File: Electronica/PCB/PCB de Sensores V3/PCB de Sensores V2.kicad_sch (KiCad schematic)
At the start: 10 parts, among them J2 Conexion Sensores, U1 ULTRASONICO1, U2 ULTRASONICO2, U3 ULTRASONICO3, U4 ULTRASONICO4, U5 ULTRASONICO5, U6 VL6180 1, U7 VL6180 2

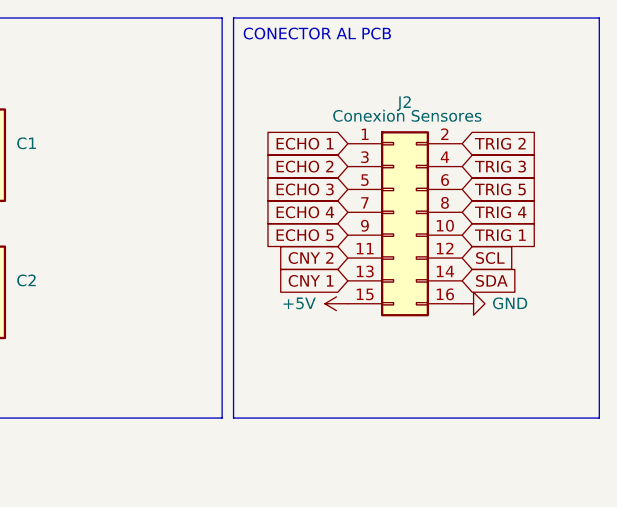
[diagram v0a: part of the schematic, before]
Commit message: Sensores V3
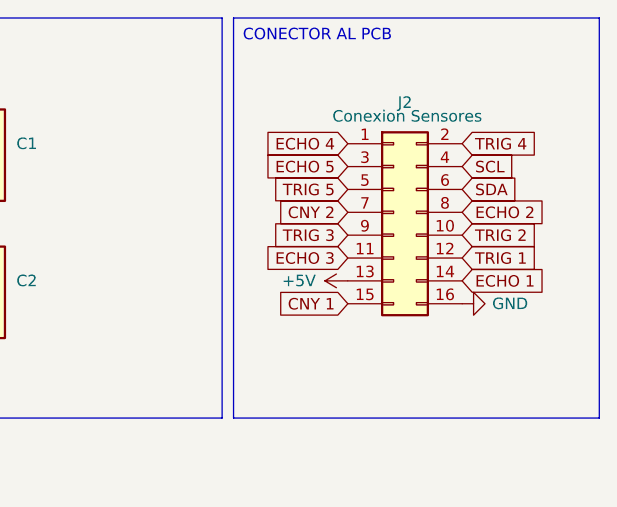
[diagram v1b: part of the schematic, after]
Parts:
- U6, U7: footprint Connector_PinHeader_2.54mm:PinHeader_1x04_P2.54mm_Horizontal -> Connector_PinHeader_2.54mm:PinHeader_1x04_P2.54mm_Vertical
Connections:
- net +5V: now also J2.13 (Pin_13); no longer J2.15 (Pin_15)
- net CNY 1: now also J2.15 (Pin_15); no longer J2.13 (Pin_13)
- net CNY 2: now also J2.7 (Pin_7); no longer J2.11 (Pin_11)
- net ECHO 1: now also J2.14 (Pin_14); no longer J2.1 (Pin_1)
- net ECHO 2: now also J2.8 (Pin_8); no longer J2.3 (Pin_3)
- net ECHO 3: now also J2.11 (Pin_11); no longer J2.5 (Pin_5)
- net ECHO 4: now also J2.1 (Pin_1); no longer J2.7 (Pin_7)
- net ECHO 5: now also J2.3 (Pin_3); no longer J2.9 (Pin_9)
- net SCL: now also J2.4 (Pin_4); no longer J2.12 (Pin_12)
- net SDA: now also J2.6 (Pin_6); no longer J2.14 (Pin_14)
- net TRIG 1: now also J2.12 (Pin_12); no longer J2.10 (Pin_10)
- net TRIG 2: now also J2.10 (Pin_10); no longer J2.2 (Pin_2)
- net TRIG 3: now also J2.9 (Pin_9); no longer J2.4 (Pin_4)
- net TRIG 4: now also J2.2 (Pin_2); no longer J2.8 (Pin_8)
- net TRIG 5: now also J2.5 (Pin_5); no longer J2.6 (Pin_6)
